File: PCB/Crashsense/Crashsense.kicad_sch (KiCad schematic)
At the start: 0 parts

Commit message: pushing KICAD flies PCB schematic
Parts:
- added C1, C2, C4, C5: 10uF, symbol Device:C
- added C3: 1uF, symbol Device:C
- added C6: 100nF, symbol Device:C
- added D1: RLED, symbol Device:LED
- added D2: GLED, symbol Device:LED
- added J1: u-blox NEO-M8N, symbol Connector:Conn_01x04_Socket
- added J2: Micro_SD_Card_Det1, symbol Connector:Micro_SD_Card_Det1
- added J3: BATTERY_CONNECTOR, symbol Connector:Conn_01x02_Socket
- added P1: USB_C_Plug_USB2.0, symbol Connector:USB_C_Plug_USB2.0
- added R1: 5.1KR, symbol Device:R
- added R10, R11, R5, R6, R7, R8, R9: 10KR, symbol Device:R
- added R2: 1.2KR, symbol Device:R
- added R3, R4: 1kR, symbol Device:R
- added U1: ESP32-S3-WROOM-1, RF_Module:ESP32-S3-WROOM-1, symbol RF_Module:ESP32-S3-WROOM-1
- added U2: ADXL377, ADXL377:LFCSP-16-3X3, symbol ADXL377:ADXL377
- added U3: BMM150, Package_CSP:WLCSP-12_1.56x1.56mm_P0.4mm, symbol Sensor_Magnetic:BMM150
- added U4: DS3231M, Package_SO:SOIC-16W_7.5x10.3mm_P1.27mm, symbol Timer_RTC:DS3231M
- added U5: BMI270, BMI270:XDCR_BMI270, symbol BMI270:BMI270
- added U6: TP4056-42-ESOP8, Package_SO:SOIC-8-1EP_3.9x4.9mm_P1.27mm_EP2.41x3.3mm_ThermalVias, symbol Battery_Management:TP4056-42-ESOP8
- added U7: ME6211C10M5, Package_TO_SOT_SMD:SOT-23-5, symbol Regulator_Linear:ME6211C10M5
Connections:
- new net: R2.1, U6.2 (PROG)
- new net: D1.1 (K), U6.6 (~{STDBY})
- new net: D2.1 (K), U6.7 (~{CHRG})
- new net: P1.A5 (CC), R1.2
- new net: D2.2 (A), R4.2
- new net: U4.10 (GND), U4.11 (GND), U4.12 (GND), U4.13 (GND), U4.5 (GND), U4.6 (GND), U4.7 (GND), U4.8 (GND), U4.9 (GND)
- new net: U3.C5 (GND), U3.E1 (GND), U3.E3 (GND)
- new net: D1.2 (A), R3.2
- new net: U1.1 (GND), U1.40 (GND), U1.41 (GND)
- new net +5V_USB: C1.1, P1.A4 (VBUS), P1.A9 (VBUS), P1.B4 (VBUS), P1.B9 (VBUS), R3.1, R4.1, U6.4 (V_{CC}), U6.8 (CE)
- new net 3V3: C4.1, C5.1, C6.1, J1.1 (Pin_1), J2.4 (VDD), R10.2, R11.2, R5.2, R6.2, R7.2, R8.2, R9.2, U7.5 (V_{OUT})
- new net DAT1: J2.8 (DAT1), R10.1
- new net DAT2: J2.1 (DAT2), R9.1
- new net GND: C1.2, C2.2, C3.2, C4.2, C5.2, C6.2, J1.2 (Pin_2), J2.10 (SHIELD), J2.6 (VSS), J3.2 (Pin_2), P1.A1 (GND), P1.A12 (GND), P1.B1 (GND), P1.B12 (GND), P1.S1 (SHIELD), R1.1, R2.2, U6.1 (TEMP), U6.3 (GND), U6.9 (EPAD), U7.2 (V_{SS})
- new net GPS_RX: J1.4 (Pin_4)
- new net GPS_TX: J1.3 (Pin_3)
- new net SD_CS: J2.2 (DAT3/CD), R8.1
- new net SD_DET: J2.9 (DET), R11.1
- new net SD_MISO: J2.7 (DAT0), R5.1
- new net SD_MOSI: J2.3 (CMD), R7.1
- new net SD_SCK: J2.5 (CLK), R6.1
- new net USB_D+: P1.A6 (D+), U1.14 (USB_D+)
- new net USB_D-: P1.A7 (D-), U1.13 (USB_D-)
- new net VBAT: C2.1, C3.1, J3.1 (Pin_1), U6.5 (BAT), U7.1 (V_{IN}), U7.3 (CE)

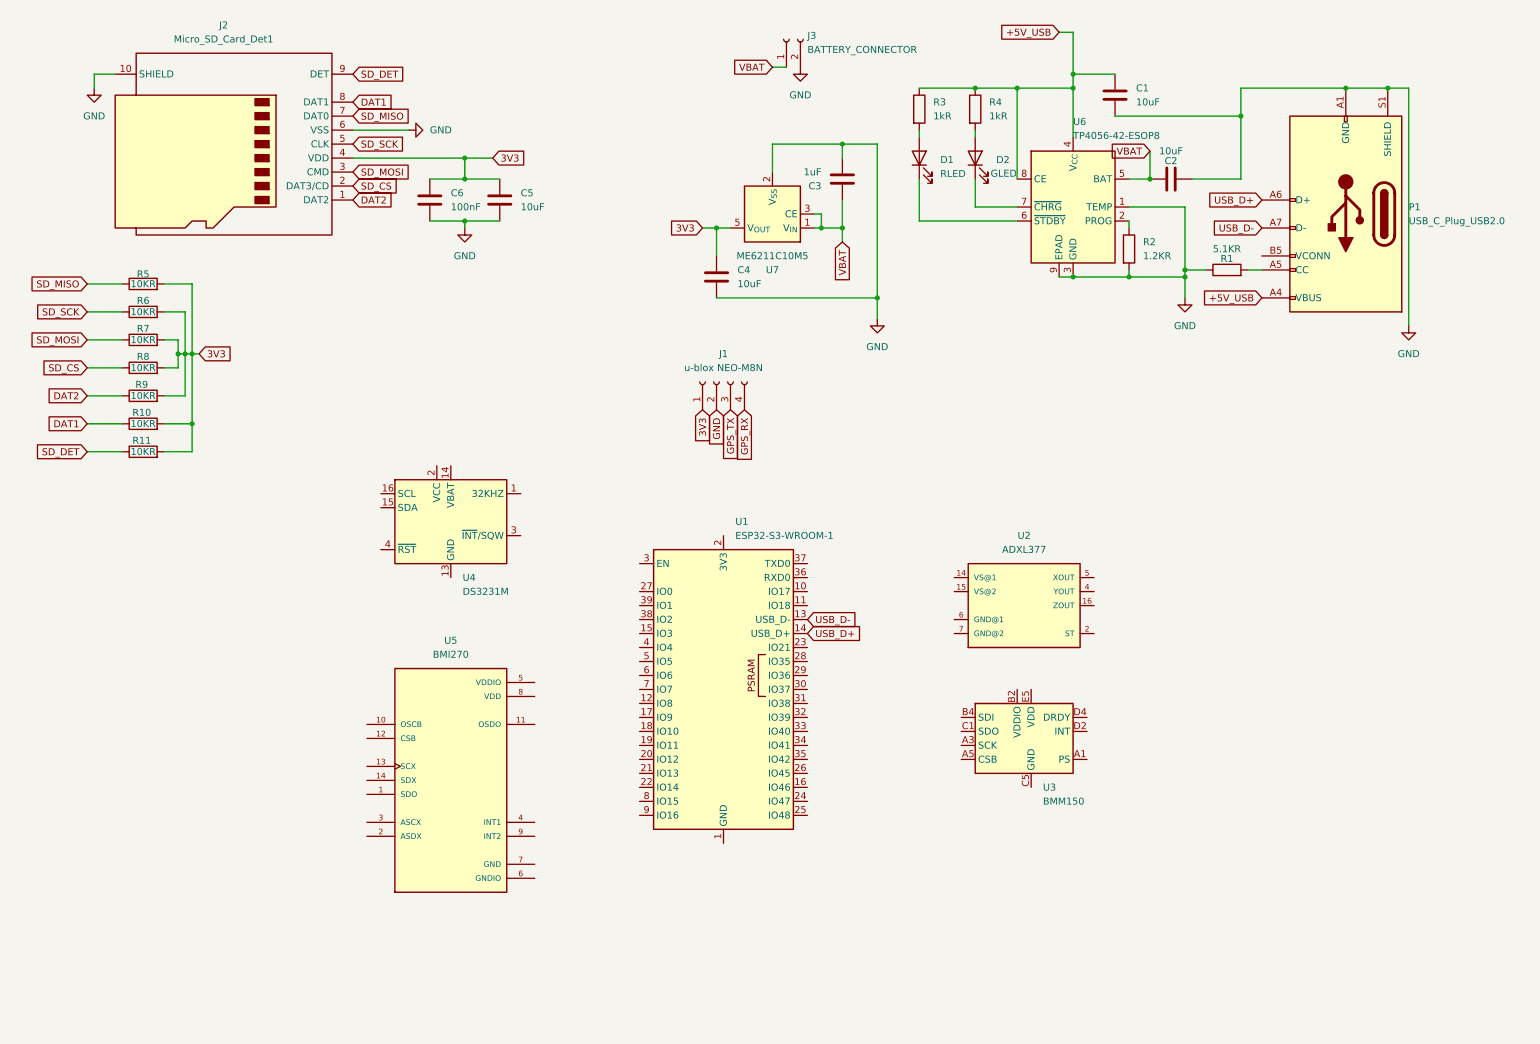
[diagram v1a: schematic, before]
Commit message: progressed on PCB and journalled for today
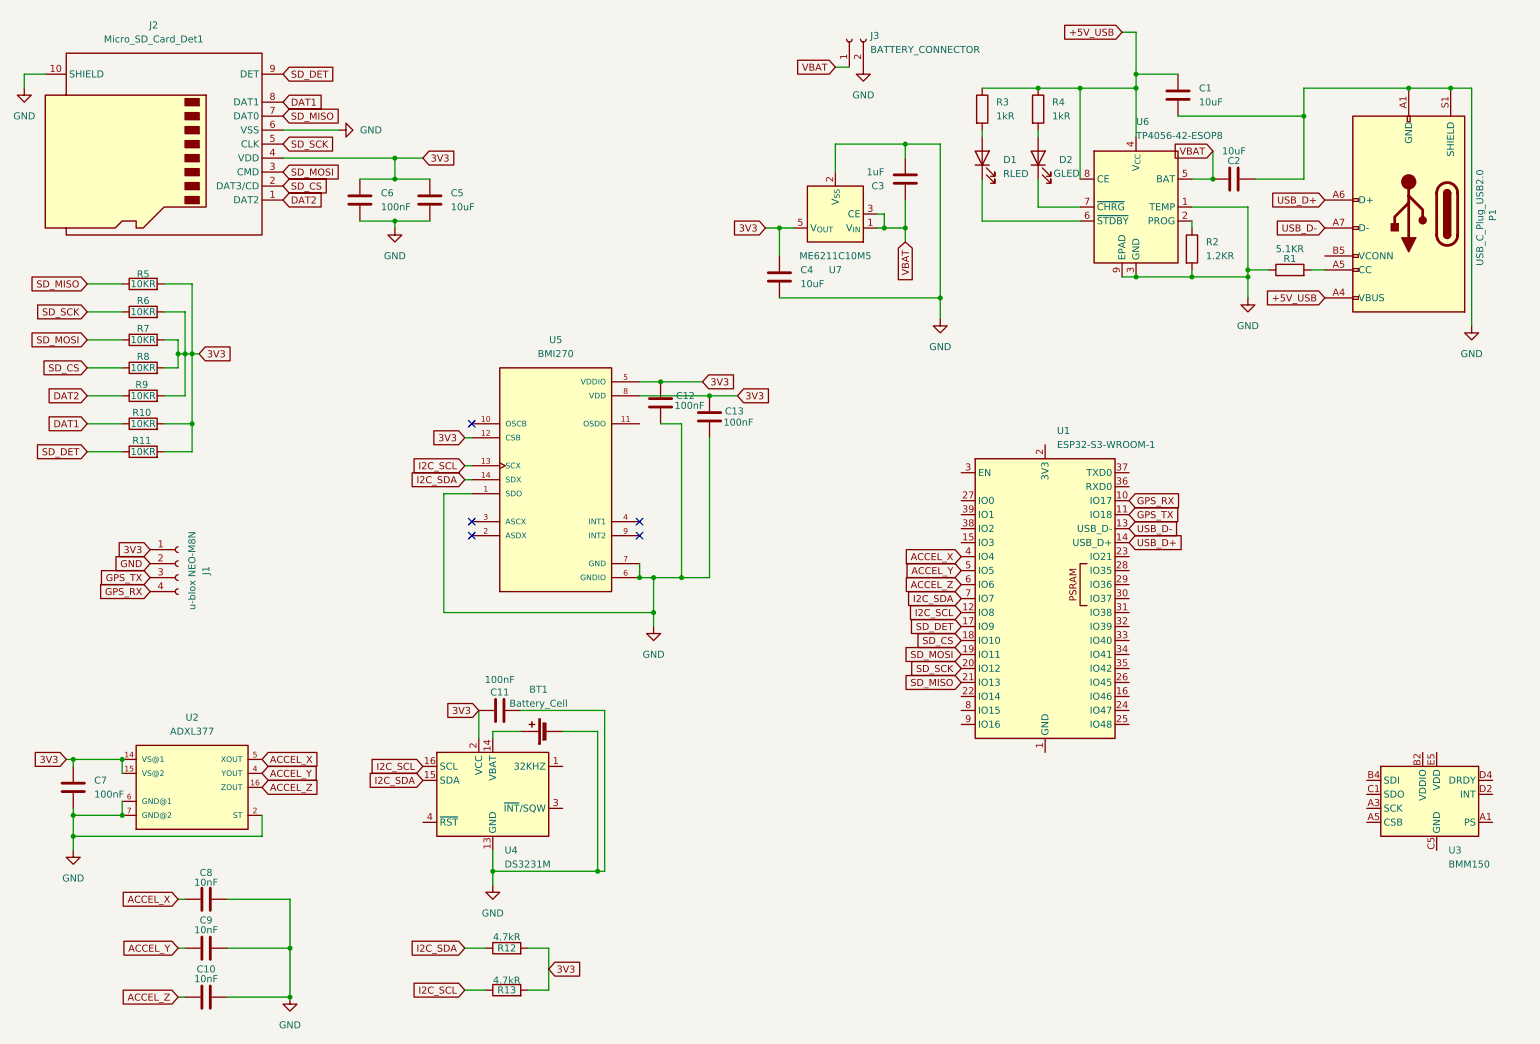
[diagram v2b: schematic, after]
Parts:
- added BT1: Battery_Cell, symbol Device:Battery_Cell
- added C10, C8, C9: 10nF, symbol Device:C
- added C11, C12, C13, C7: 100nF, symbol Device:C
- added R12, R13: 4.7kR, symbol Device:R
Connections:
- net 3V3: now also U2.14 (VS@1), U2.15 (VS@2), U4.2 (VCC), U5.12 (CSB), U5.5 (VDDIO), U5.8 (VDD), C11.1, C12.1, C13.1, C7.1, R12.2, R13.2
- net GND: now also U2.2 (ST), U2.6 (GND@1), U2.7 (GND@2), U4.10 (GND), U4.11 (GND), U4.12 (GND), U4.13 (GND), U4.5 (GND), U4.6 (GND), U4.7 (GND), U4.8 (GND), U4.9 (GND), U5.1 (SDO), U5.6 (GNDIO), U5.7 (GND), BT1.2 (-), C10.2, C11.2, C12.2, C13.2, C7.2, C8.2, C9.2
- net GPS_RX: now also U1.10 (IO17)
- net GPS_TX: now also U1.11 (IO18)
- net SD_CS: now also U1.18 (IO10)
- net SD_DET: now also U1.17 (IO9)
- net SD_MISO: now also U1.21 (IO13)
- net SD_MOSI: now also U1.19 (IO11)
- net SD_SCK: now also U1.20 (IO12)
- net I2C_SCL: now reaches U5.13 (SCX)
- net I2C_SCL: now also U1.12 (IO8), U4.16 (SCL), R13.1
- net I2C_SDA: now reaches U5.14 (SDX)
- net I2C_SDA: now also U1.7 (IO7), U4.15 (SDA), R12.1
- net at U4.14 (VBAT): now also BT1.1 (+)
- net ACCEL_Z: now reaches U2.16 (ZOUT)
- net ACCEL_Z: now also U1.6 (IO6), C10.1
- net ACCEL_Y: now reaches U2.4 (YOUT)
- net ACCEL_Y: now also U1.5 (IO5), C9.1
- net ACCEL_X: now reaches U2.5 (XOUT)
- net ACCEL_X: now also U1.4 (IO4), C8.1
- no-connect marks 0 -> 5
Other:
- moved on the sheet: C1, C2, C3, C4, C5, C6, D1, D2, J1, J2, J3, P1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

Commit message: finished PCB and journalled
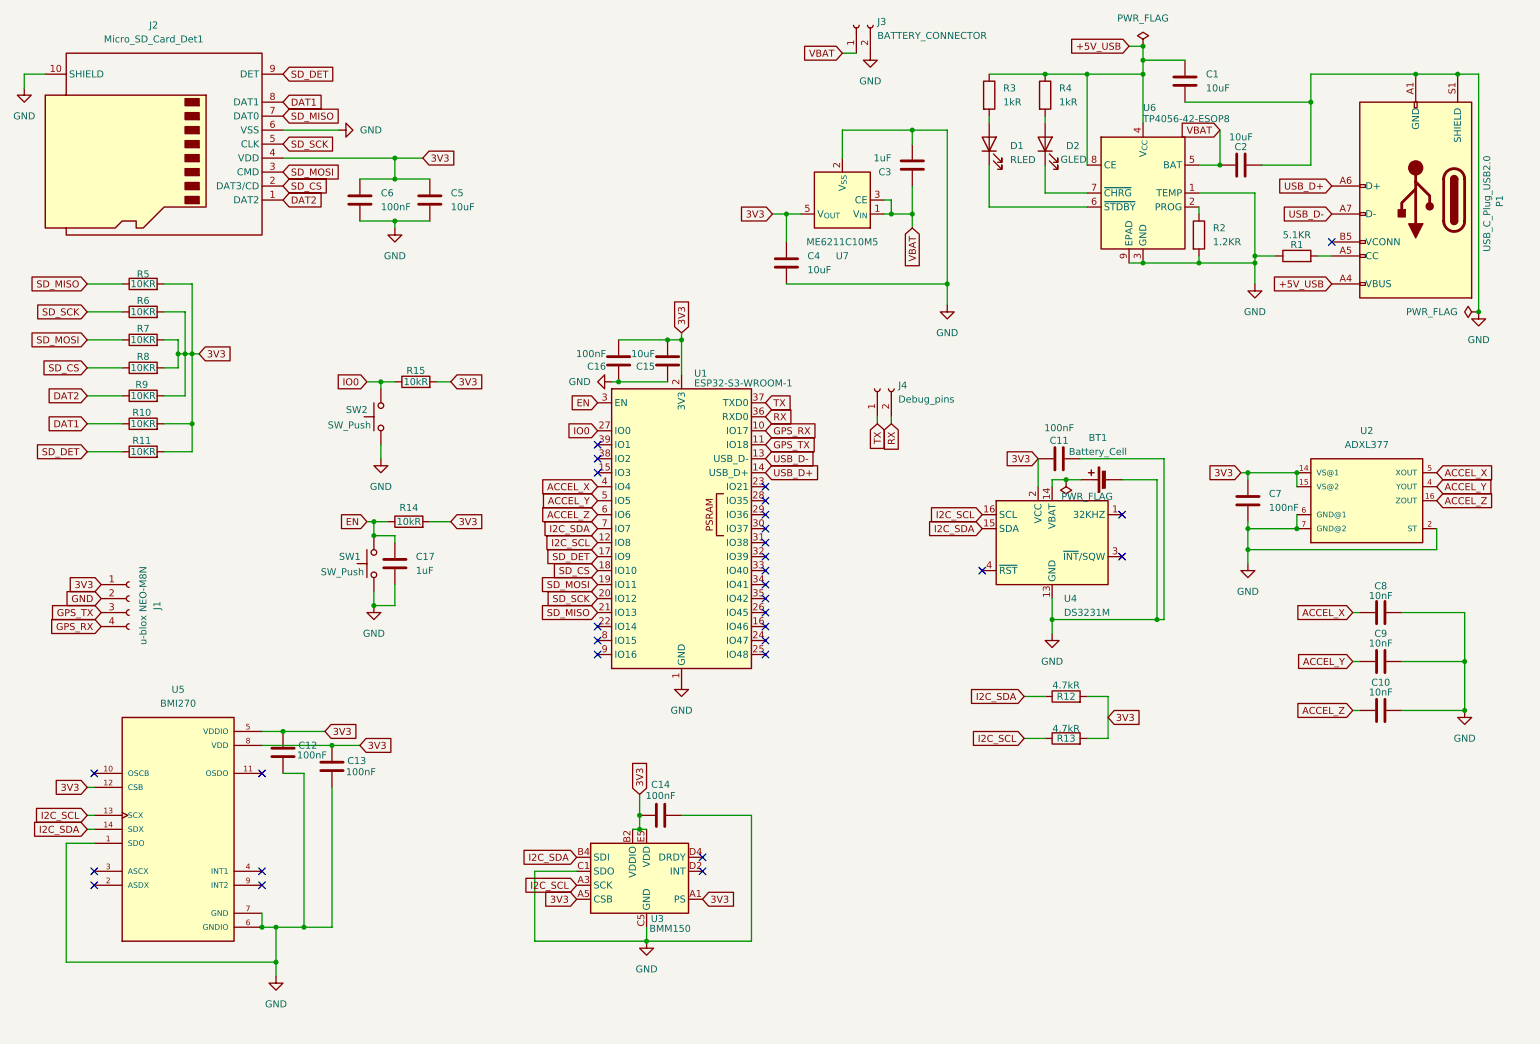
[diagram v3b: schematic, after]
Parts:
- added C14, C16: 100nF, Capacitor_SMD:C_0805_2012Metric, symbol Device:C
- added C15: 10uF, Capacitor_SMD:C_0805_2012Metric, symbol Device:C
- added C17: 1uF, Capacitor_SMD:C_0805_2012Metric, symbol Device:C
- added J4: Debug_pins, Connector_PinHeader_2.54mm:PinHeader_1x02_P2.54mm_Vertical, symbol Connector:Conn_01x02_Socket
- added R14, R15: 10kR, Resistor_SMD:R_0805_2012Metric, symbol Device:R
- added SW1, SW2: SW_Push, Button_Switch_SMD:SW_SPST_SKQG_WithStem, symbol Switch:SW_Push
- BT1: footprint (none) -> Battery:BatteryHolder_Keystone_3034_1x20mm
- C1, C10, C11, C12, C13, C2, C3, C4, C5, C6, C7, C8, C9: footprint (none) -> Capacitor_SMD:C_0805_2012Metric
- D1, D2: footprint (none) -> LED_SMD:LED_0805_2012Metric
- J1: footprint (none) -> Connector_PinHeader_2.54mm:PinHeader_1x04_P2.54mm_Vertical
- J2: footprint (none) -> Connector_Card:microSD_HC_Hirose_DM3D-SF
- J3: footprint (none) -> Connector_JST:JST_PH_B2B-PH-K_1x02_P2.00mm_Vertical
- P1: footprint (none) -> Connector_USB:USB_C_Receptacle_HRO_TYPE-C-31-M-12
- R1, R10, R11, R12, R13, R2, R3, R4, R5, R6, R7, R8, R9: footprint (none) -> Resistor_SMD:R_0805_2012Metric
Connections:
- net 3V3: now also U1.2 (3V3), U3.A1 (PS), U3.A5 (CSB), U3.B2 (VDDIO), U3.E5 (VDD), C14.1, C15.2, C16.2, R14.2, R15.2
- net GND: now also U1.1 (GND), U1.40 (GND), U1.41 (GND), U3.C1 (SDO), U3.C5 (GND), U3.E1 (GND), U3.E3 (GND), C14.2, C15.1, C16.1, C17.2, SW1.1, SW2.1
- net I2C_SCL: now also U3.A3 (SCK)
- net I2C_SDA: now also U3.B4 (SDI)
- net IO0: now reaches U1.27 (IO0)
- net IO0: now also R15.1, SW2.2
- net EN: now reaches U1.3 (EN)
- net EN: now also C17.1, R14.1, SW1.2
- net RX: now reaches U1.36 (RXD0)
- net RX: now also J4.2 (Pin_2)
- net TX: now reaches U1.37 (TXD0)
- net TX: now also J4.1 (Pin_1)
- no-connect marks 5 -> 31
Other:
- moved on the sheet: BT1, C1, C10, C11, C12, C13, C2, C3, C4, C7, C8, C9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
